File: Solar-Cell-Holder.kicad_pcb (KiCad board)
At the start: 2 copper layers, 84.3 x 68.6 mm, 3 parts, among them J1 Conn_01x01_Female, U1 XTJ

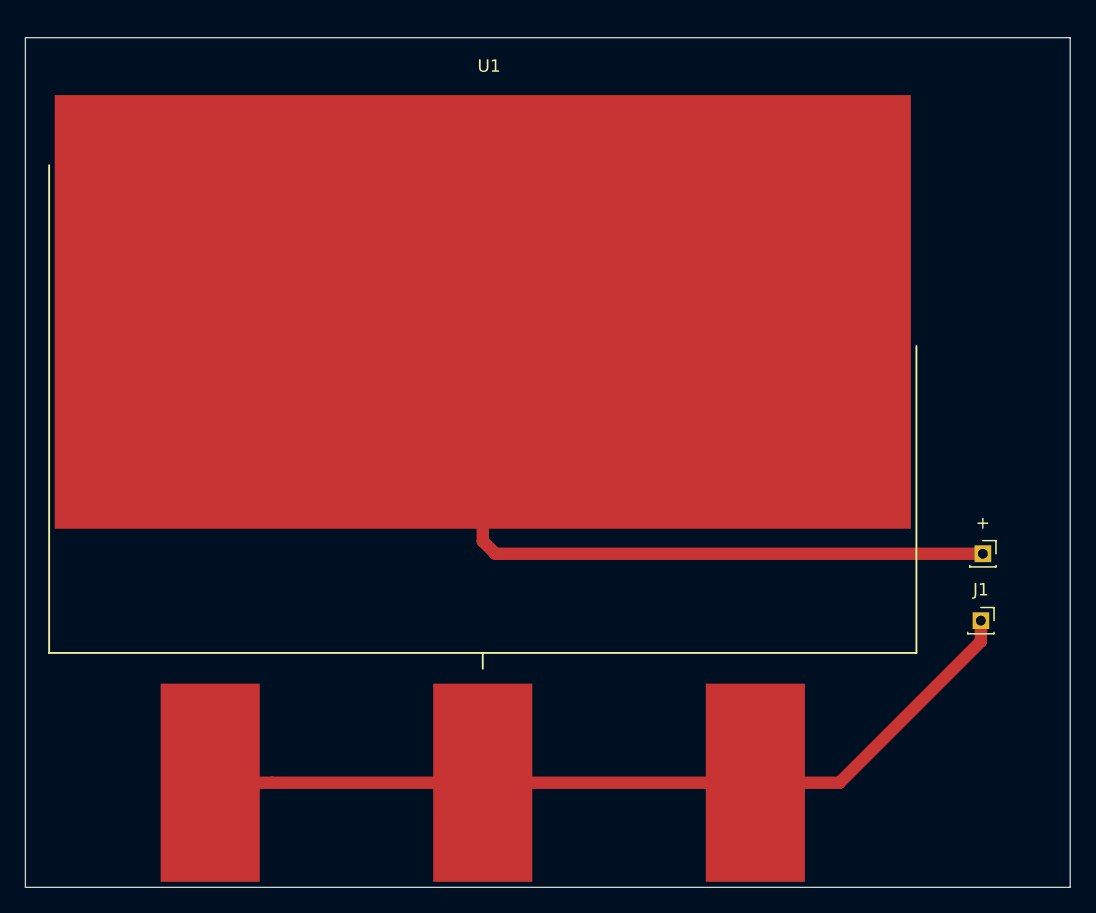
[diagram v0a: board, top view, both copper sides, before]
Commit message: finished
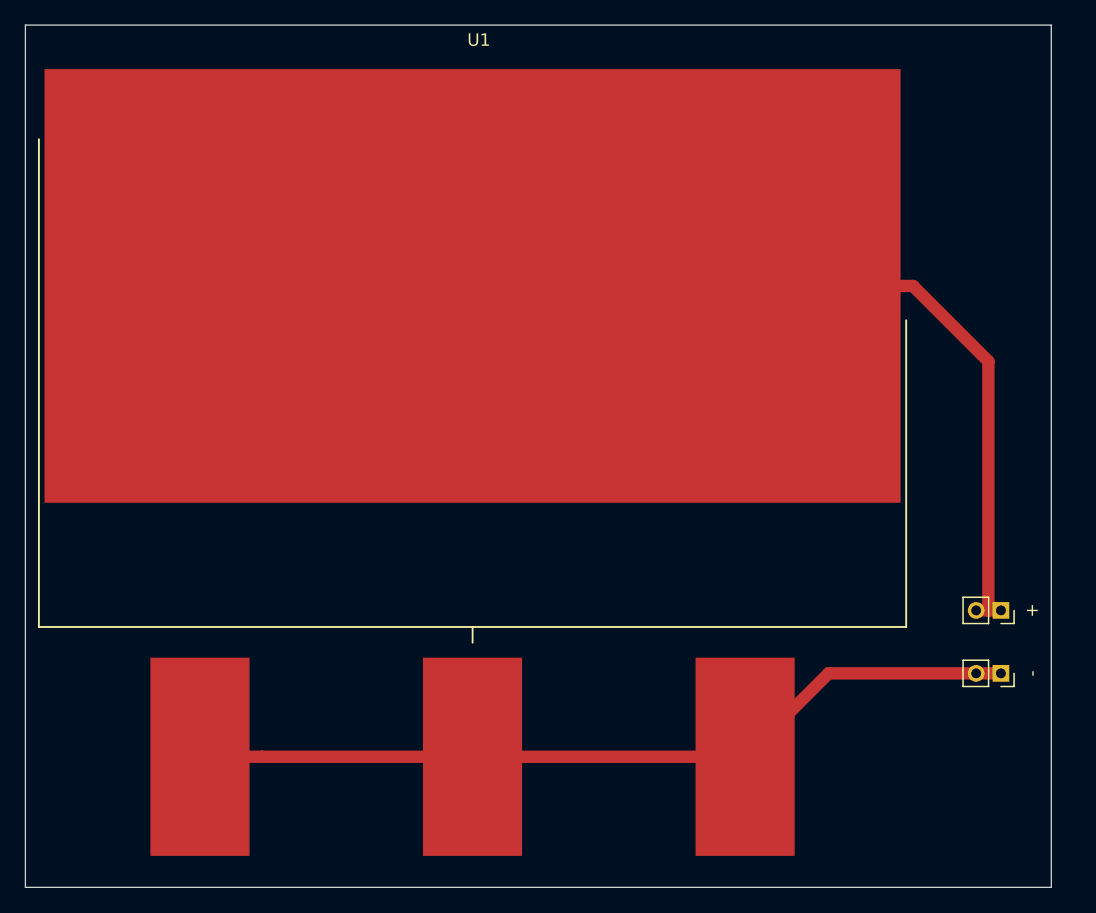
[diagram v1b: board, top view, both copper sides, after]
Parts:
- removed the + at (178.9, 74.2)
- removed J1: Conn_01x01_Female, Connector_PinSocket_2.00mm:PinSocket_1x01_P2.00mm_Vertical
- added +: Conn_01x02_Female, Connector_PinSocket_2.00mm:PinSocket_1x02_P2.00mm_Vertical, F.Cu at (180.3, 78.7)
- added -: Conn_01x02_Female, Connector_PinSocket_2.00mm:PinSocket_1x02_P2.00mm_Vertical, F.Cu at (180.3, 83.8)
- moved U1 2.25 mm to (137.7, 70.6)
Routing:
- net Net-(J2-Pad1): track 59.3 -> 81.7 mm
- net Net-(J1-Pad1): track 68.6 -> 72.1 mm
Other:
- board size 84.3 x 68.6 mm -> 82.8 x 69.6 mm
